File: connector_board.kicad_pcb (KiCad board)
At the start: 2 copper layers, 120 x 62 mm, 17 parts, among them J1 Screw Terminal Block 5.00 mm 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, J10 Screw Terminal Block 3.50 mm 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, J11 2s-tc2030-NL, J12 TC2050 With UART NL, J13 1-350942-0, J2 2s_cortex-m-10-pin, J3 2s-tc2030, J4 2s_cortex-m-10-pin, J5 1757242, J6 S3B-ZR-SM4A-TF, J7 JST S3B-XH-A, J8 JST S3B-PH-K-S, J9 JST SM03B-SRSS-TB

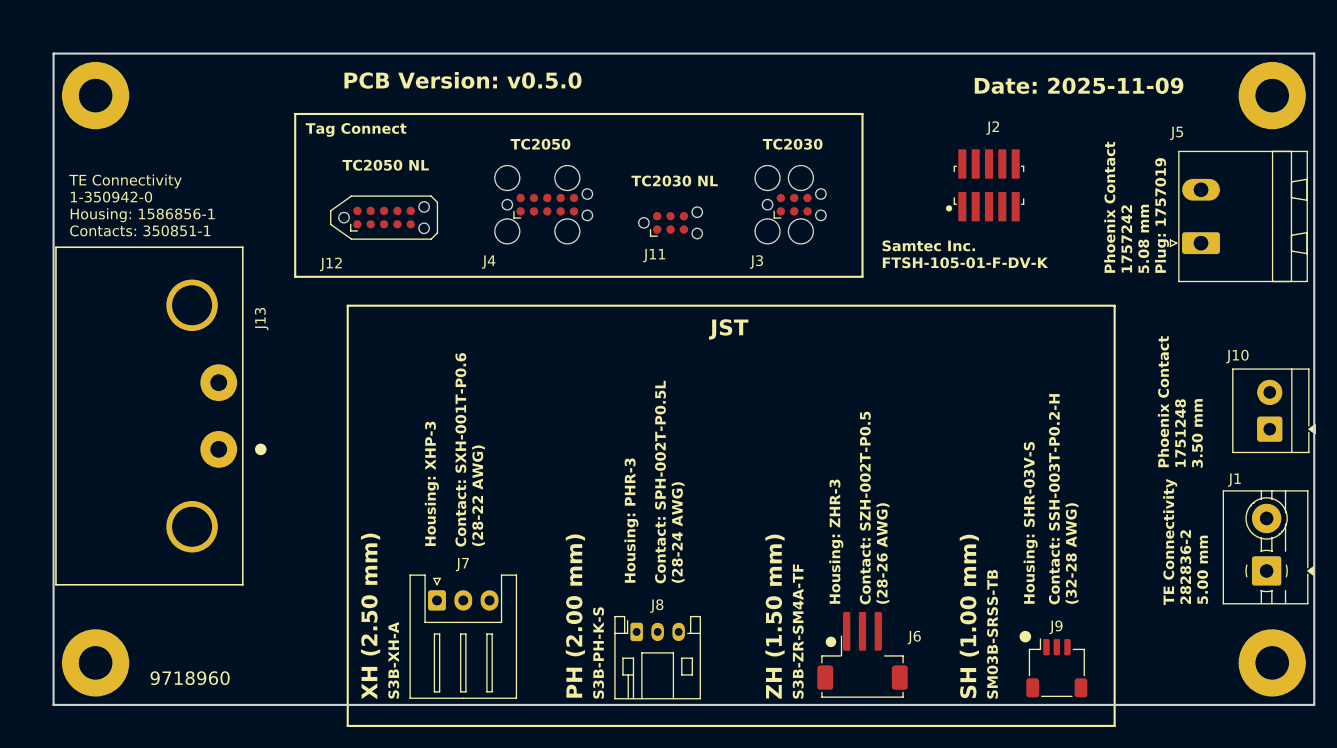
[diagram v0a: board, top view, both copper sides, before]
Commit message: fix: small improvements I guess
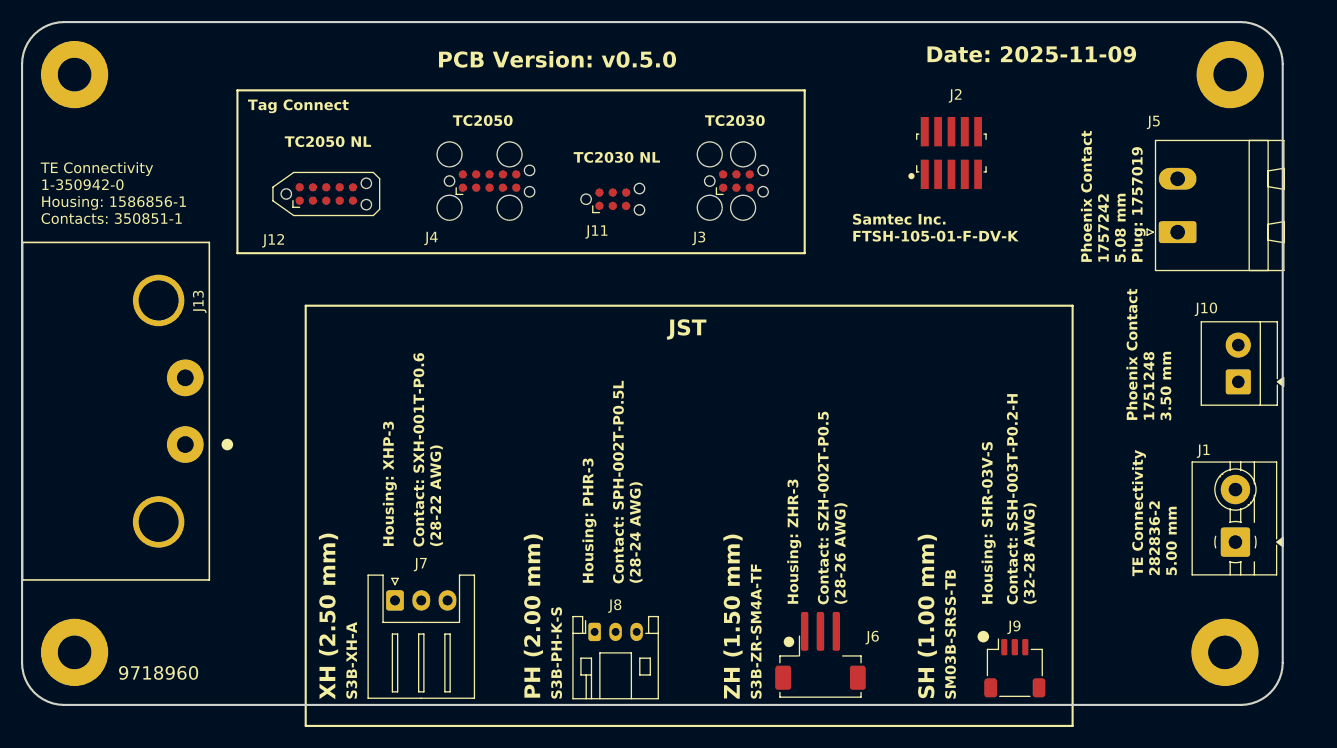
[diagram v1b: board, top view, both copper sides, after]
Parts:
- moved J11 5.94 mm to (111.2, 46.9)
- moved J12 5.94 mm to (84.0, 46.4)
- moved J3 5.94 mm to (123.0, 45.1)
- moved J4 5.94 mm to (99.5, 45.1)
- moved J10 5.41 mm to (170.8, 64.2)
- moved J2 4.72 mm to (143.5, 42.5)
- moved H2 4.61 mm to (169.5, 90.0)
- moved H3 4.47 mm to (170.0, 35.0)
- moved J1 4.05 mm to (170.5, 79.5)
- moved J6 4.00 mm to (131.0, 91.0)
- moved J7 4.00 mm to (90.5, 85.1)
- moved J8 4.00 mm to (109.5, 88.0)
- moved J9 4.00 mm to (149.5, 91.5)
- moved J13 3.21 mm to (70.5, 70.2)
- moved H4 2.83 mm to (60.0, 35.0)
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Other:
- board size 120 x 62 mm -> 120 x 65 mm
